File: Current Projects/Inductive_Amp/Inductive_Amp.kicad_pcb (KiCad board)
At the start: 2 copper layers, 10 parts, among them J1 Conn_01x03, J2 Conn_01x03, U1 NA555D, U2 74LS14, U3 TLV2372

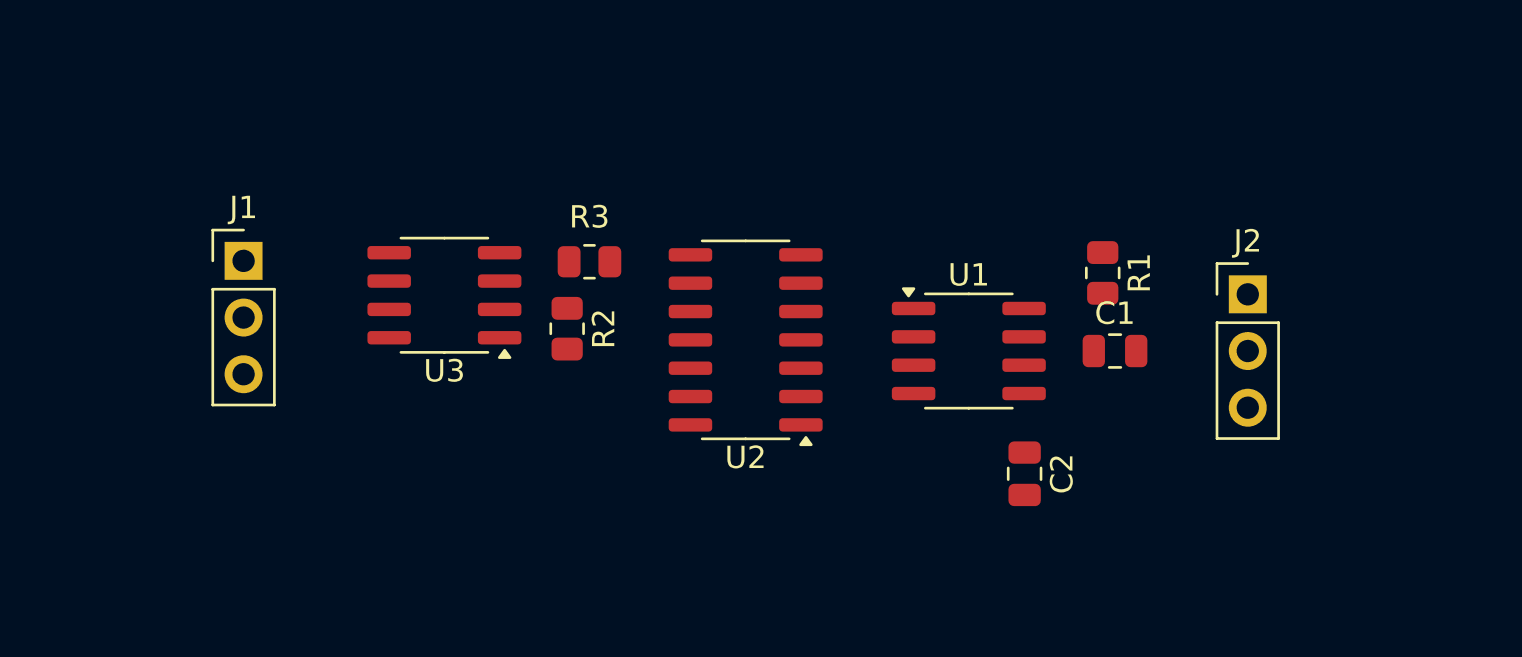
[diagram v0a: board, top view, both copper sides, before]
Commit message: Inductive PCB!
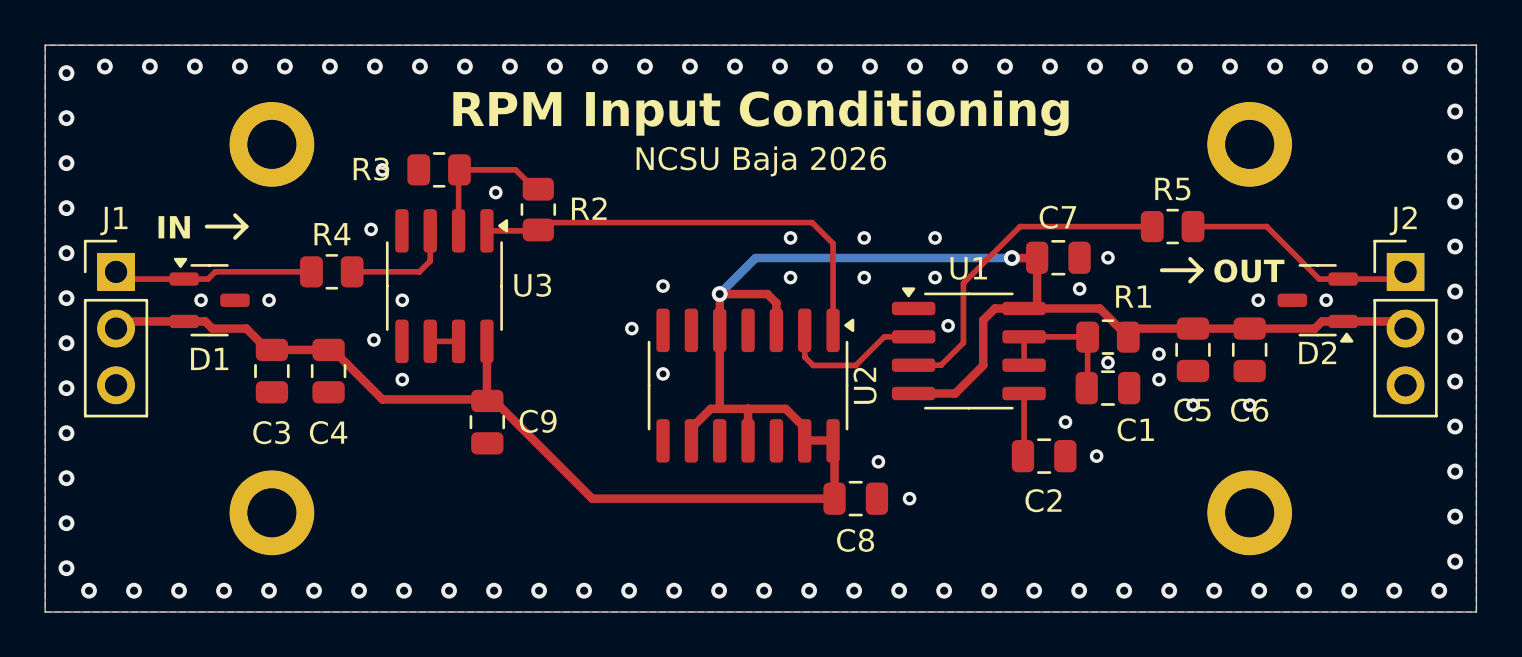
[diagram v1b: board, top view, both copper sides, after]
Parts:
- added C3: 0.1u, Capacitor_SMD:C_0805_2012Metric, F.Cu at (128.3, 88.9)
- added C4: 1u, Capacitor_SMD:C_0805_2012Metric, F.Cu at (130.8, 88.9)
- added C5: 1u, Capacitor_SMD:C_0805_2012Metric, F.Cu at (169.5, 87.9)
- added C6: 0.1u, Capacitor_SMD:C_0805_2012Metric, F.Cu at (172.1, 87.9)
- added C7: 0.1u, Capacitor_SMD:C_0805_2012Metric, F.Cu at (163.5, 83.8)
- added C8: 0.1u, Capacitor_SMD:C_0805_2012Metric, F.Cu at (154.4, 94.6)
- added C9: 0.1u, Capacitor_SMD:C_0805_2012Metric, F.Cu at (137.9, 91.2)
- added D1: PESD5V0S2BT, Package_TO_SOT_SMD:SOT-23-3, F.Cu at (125.5, 85.7)
- added D2: PESD5V0S2BT, Package_TO_SOT_SMD:SOT-23-3, F.Cu at (175.1, 85.7)
- added H1: M2, MountingHole:MountingHole_2.2mm_M2_DIN965_Pad, F.Cu at (128.3, 78.7)
- added H2: M2, MountingHole:MountingHole_2.2mm_M2_DIN965_Pad, F.Cu at (128.3, 95.2)
- added H3: M2, MountingHole:MountingHole_2.2mm_M2_DIN965_Pad, F.Cu at (172.1, 78.7)
- added H4: M2, MountingHole:MountingHole_2.2mm_M2_DIN965_Pad, F.Cu at (172.1, 95.2)
- added R4: 1k, Resistor_SMD:R_0805_2012Metric, F.Cu at (131.0, 84.5)
- added R5: 1k, Resistor_SMD:R_0805_2012Metric, F.Cu at (168.6, 82.4)
- J1: value Conn_01x03 -> INPUT
- J2: value Conn_01x03 -> OUTPUT
- R2: value 1k -> 15k
- R3: value 200 -> 10k
- moved R3 7.90 mm to (135.8, 79.9), turned to 180 degrees
- moved J2 7.14 mm to (179.1, 84.5)
- moved J1 5.74 mm to (121.3, 84.5)
- moved R2 5.49 mm to (140.2, 81.7)
- moved R1 2.89 mm to (165.7, 87.4), turned to 180 degrees
- moved U2 2.05 mm to (149.6, 89.5), turned to -90 degrees
- moved C1 1.69 mm to (165.7, 89.7)
- moved C2 1.18 mm to (162.9, 92.7), turned to 0 degrees
- moved U3 0.41 mm to (136.0, 85.1), turned to -90 degrees
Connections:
- U1 pad 3: /OUT -> Net-(U1-Q)
- U2 pad 1: Net-(U2-Pad1) -> Net-(R2-Pad2)
- U2 pad 10: (no net) -> unconnected-(U2-Pad10)
- U2 pad 11: (no net) -> +5V
- U2 pad 12: (no net) -> unconnected-(U2-Pad12)
- U2 pad 13: (no net) -> +5V
- U2 pad 3: Net-(R2-Pad2) -> +5V
- U2 pad 4: Net-(U2-Pad1) -> unconnected-(U2-Pad4)
- U2 pad 5: (no net) -> +5V
- U2 pad 6: (no net) -> unconnected-(U2-Pad6)
- U2 pad 8: (no net) -> unconnected-(U2-Pad8)
- U2 pad 9: (no net) -> +5V
- U3 pad 3: /Vin -> Net-(U3A-+)
- U3 pad 4: (no net) -> GND
- U3 pad 5: (no net) -> GND
- U3 pad 6: (no net) -> Net-(U3B--)
- U3 pad 7: (no net) -> Net-(U3B--)
- U3 pad 8: (no net) -> +5V
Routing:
- net +5V: track 0.00 -> 103.1 mm, vias 0 -> 2
- net Net-(R2-Pad2): track 0.00 -> 19.9 mm
- net Net-(U1-Q): track 0.00 -> 14.8 mm
- net /OUT: track 0.00 -> 10.6 mm
- net /Vin: track 0.00 -> 9.03 mm
- net Net-(U1-TR): track 0.00 -> 6.76 mm
- net Net-(U3A--): track 0.00 -> 6.64 mm
- net Net-(U1-DIS): track 0.00 -> 6.42 mm
- net Net-(U3A-+): track 0.00 -> 5.05 mm
- net Net-(U1-CV): track 0.00 -> 2.83 mm
- net Net-(U3B--): track 0.00 -> 1.27 mm
- net GND: vias 0 -> 116
- added copper zone on B.Cu, net GND
- added copper zone on F.Cu, net GND
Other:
- board outline added: 64.1 x 25.4 mm
- board text added: "IN"
- board text added: "NCSU Baja 2026"
- board text added: "OUT"
- board text added: "RPM Input Conditioning"
